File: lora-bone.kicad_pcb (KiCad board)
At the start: 2 copper layers, 30 x 100 mm, 23 parts, among them J1 Analog IN, J10 GS2, J11 GS2, J12 GS2, J13 GS2, J15 CONN_COAXIAL, J2 POWER, J3 Bluepill left, J4 PWM OUT, J5 SPI OUT, J6 Bluepill right, J7 I2C, J8 GPIO, J9 UART, U1 RFM95W

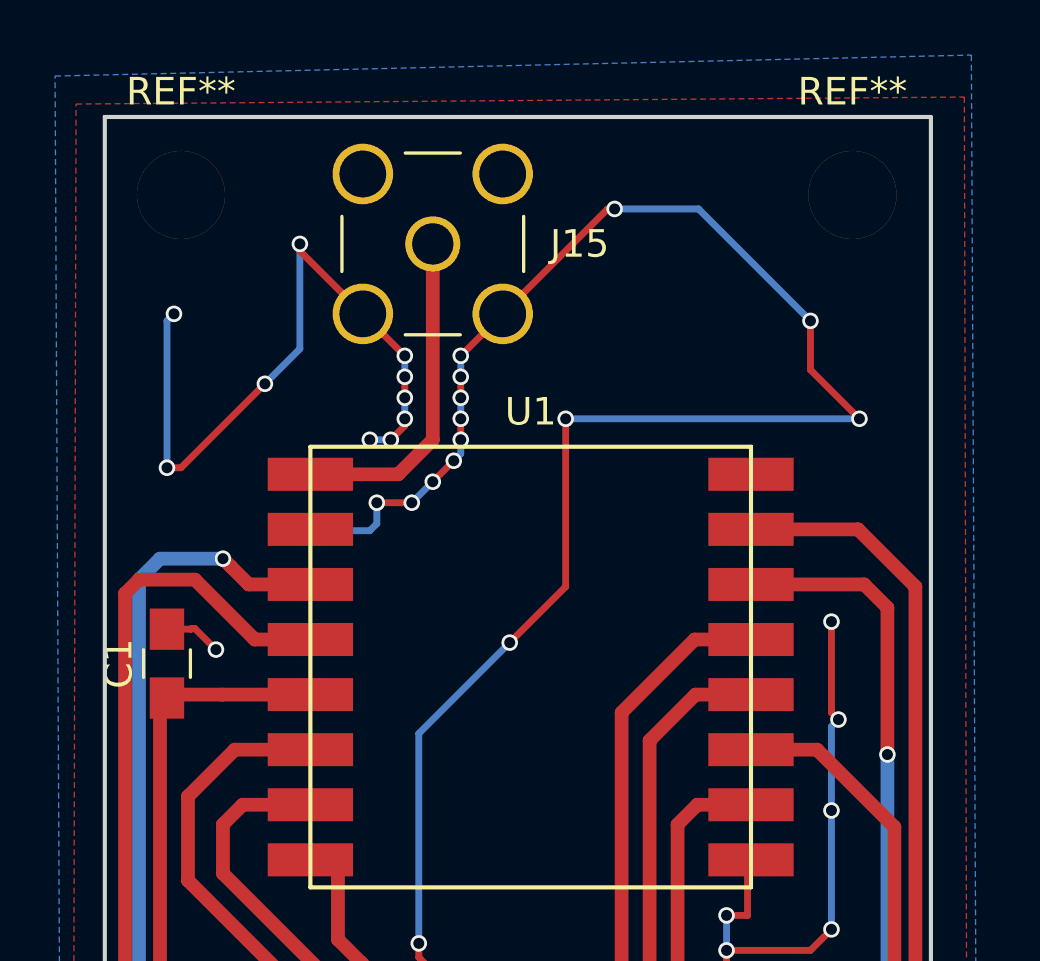
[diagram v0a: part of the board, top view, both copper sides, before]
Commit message: A few little corrections
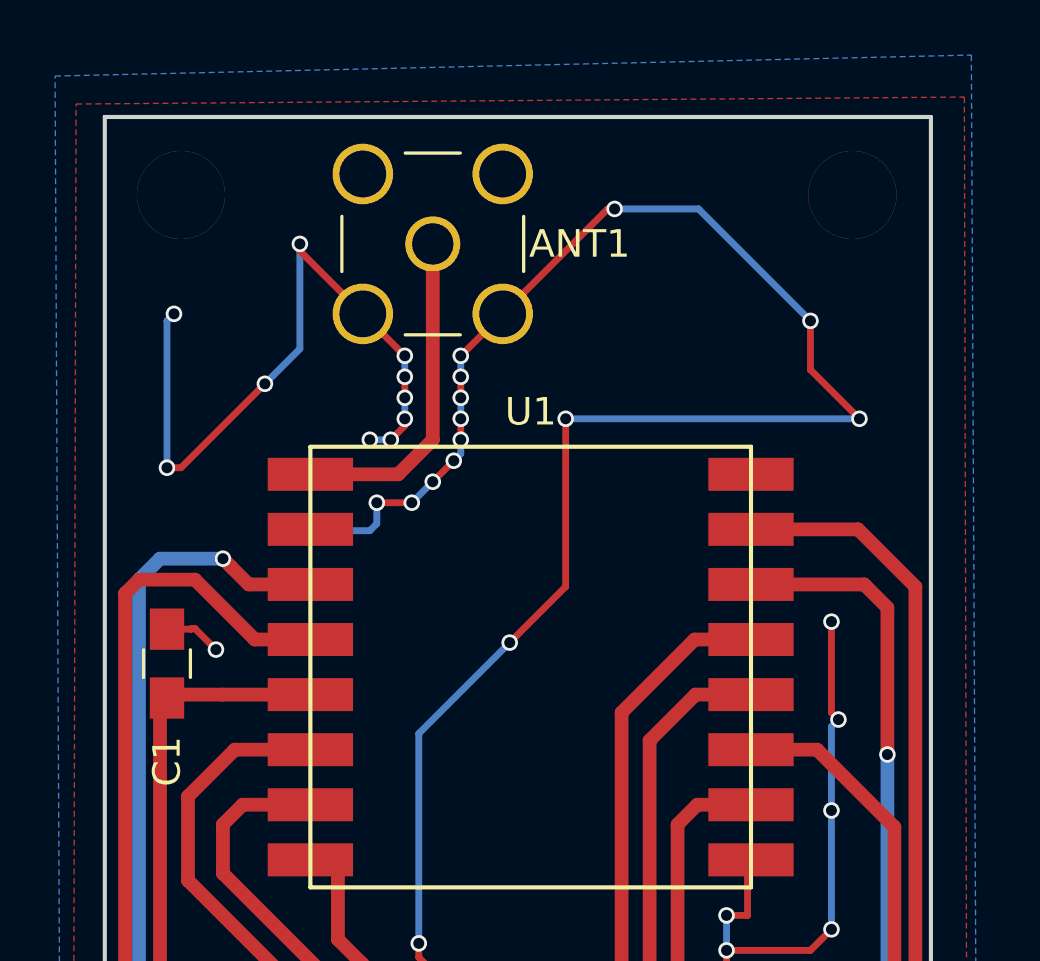
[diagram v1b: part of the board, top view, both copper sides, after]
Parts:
- renumbered J15 to ANT1
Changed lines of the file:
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@@
   (net 40 "Net-(J3-Pad17)")
   (net 41 "Net-(J6-Pad20)")
-  (net 42 "Net-(J15-Pad1)")
+  (net 42 "Net-(ANT1-Pad1)")
   (net_class Default "This is the default net class."
     (clearance 0.2)
@@
     (add_net MISO)
     (add_net MOSI)
-    (add_net "Net-(J15-Pad1)")
+    (add_net "Net-(ANT1-Pad1)")
     (add_net "Net-(J3-Pad1)")
     (add_net "Net-(J3-Pad13)")
@@
     (descr "Mounting Hole 3.2mm, no annular, M3, ISO14580")
     (tags "mounting hole 3.2mm no annular m3 iso14580")
-    (fp_text reference REF** (at 0 -3.75) (layer F.SilkS)
+    (fp_text reference REF** (at 0 -3.75) (layer F.SilkS) hide
       (effects (font (size 1 1) (thickness 0.15)))
     )
@@
     (descr "SMA pcb through hole jack")
     (tags "SMA THT Jack Straight")
-    (fp_text reference J15 (at 5.334 0) (layer F.SilkS)
+    (fp_text reference ANT1 (at 5.334 0) (layer F.SilkS)
       (effects (font (size 1 1) (thickness 0.15)))
     )
@@
       (net 3 GND))
     (pad 1 thru_hole circle (at 0 0) (size 2 2) (drill 1.5) (layers *.Cu *.Mask)
-      (net 42 "Net-(J15-Pad1)"))
+      (net 42 "Net-(ANT1-Pad1)"))
   )
   (module Capacitors_SMD:C_0805_HandSoldering (layer F.Cu)
@@
     (tags "capacitor 0805")
     (attr smd)
-    (fp_text reference C1 (at 0 -1.75 90) (layer F.SilkS)
+    (fp_text reference C1 (at -3.556 0 90) (layer F.SilkS)
       (effects (font (size 1 1) (thickness 0.15)))
     )
@@
       (net 3 GND))
     (pad 9 smd rect (at 7 -1 180) (size 3.1 1.2) (drill (offset 1 0)) (layers F.Cu F.Paste F.Mask)
-      (net 42 "Net-(J15-Pad1)"))
+      (net 42 "Net-(ANT1-Pad1)"))
     (pad 8 smd rect (at -7 -1 180) (size 3.1 1.2) (drill (offset -1 0)) (layers F.Cu F.Paste F.Mask)
       (net 3 GND))
@@
     (descr "Mounting Hole 3.2mm, no annular, M3, ISO14580")
     (tags "mounting hole 3.2mm no annular m3 iso14580")
-    (fp_text reference REF** (at 0 -3.75) (layer F.SilkS)
-      (effects (font (size 1 1) (thickness 0.15)))
-    )
+    (fp_text reference REF** (at 0 -3.75) (layer F.SilkS) hide
+      (effects (font (size 1 1) (thickness 0.15)))
+    )
